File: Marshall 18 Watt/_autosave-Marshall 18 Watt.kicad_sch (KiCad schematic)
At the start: 37 parts, among them J1 LOW, J2 HIGH, J3 Conn_01x03_Socket, J4 Heater, U1 ECC83, U2 ECC83, U3 EL84, U4 EL84

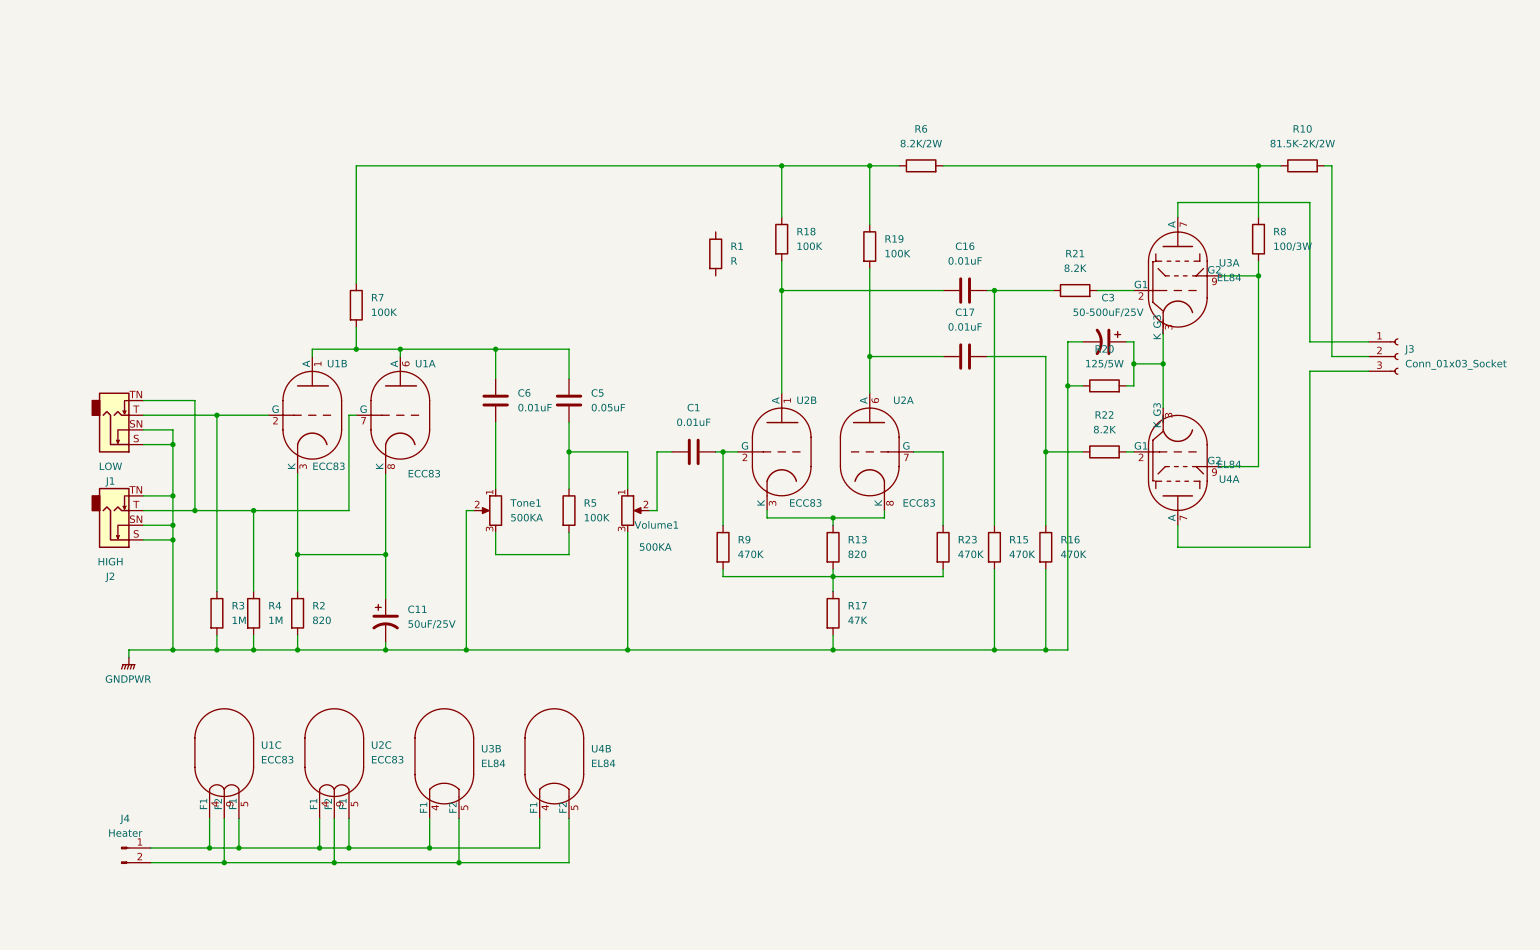
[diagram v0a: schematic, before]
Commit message: Update_17_03_25
Add sch
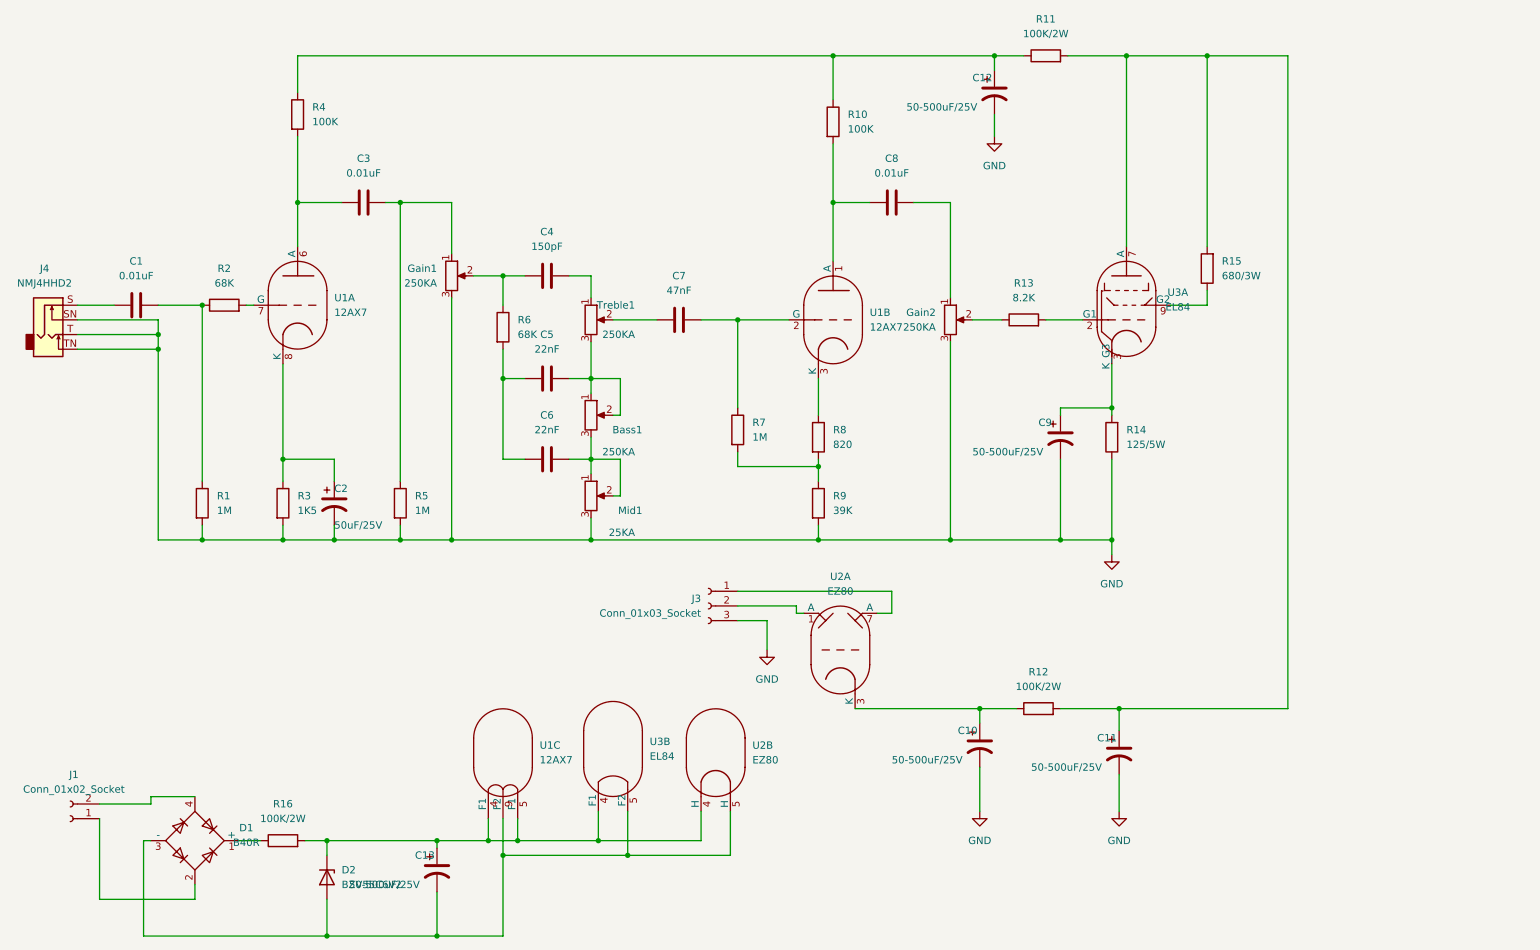
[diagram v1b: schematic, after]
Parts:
- removed C17: 0.01uF, Capacitor_THT:C_Axial_L5.1mm_D3.1mm_P10.00mm_Horizontal, symbol Device:C
- removed J1: LOW, Connector_Audio:Jack_6.35mm_Neutrik_NMJ4HCD2_Horizontal, symbol Connector_Audio:NMJ4HHD2
- removed J2: HIGH, Connector_Audio:Jack_6.35mm_Neutrik_NMJ4HCD2_Horizontal, symbol Connector_Audio:NMJ4HHD2
- removed J4: Heater, Connector_Phoenix_MC_HighVoltage:PhoenixContact_MCV_1,5_2-G-5.08_1x02_P5.08mm_Vertical, symbol Connector:Conn_01x02_Pin
- removed R1: R, Resistor_THT:R_Axial_DIN0411_L9.9mm_D3.6mm_P20.32mm_Horizontal, symbol Device:R
- removed R10: 81.5K-2K/2W, Resistor_THT:R_Axial_DIN0411_L9.9mm_D3.6mm_P20.32mm_Horizontal, symbol Device:R
- removed R15, R23: 470K, Resistor_THT:R_Axial_DIN0411_L9.9mm_D3.6mm_P20.32mm_Horizontal, symbol Device:R
- removed R19: 100K, Resistor_THT:R_Axial_DIN0411_L9.9mm_D3.6mm_P20.32mm_Horizontal, symbol Device:R
- removed R22: 8.2K, Resistor_THT:R_Axial_DIN0411_L9.9mm_D3.6mm_P20.32mm_Horizontal, symbol Device:R
- removed R4: 1M, Resistor_THT:R_Axial_DIN0411_L9.9mm_D3.6mm_P20.32mm_Horizontal, symbol Device:R
- removed U1, U2: ECC83, Valve:Valve_Noval_P, symbol Valve:ECC83
- removed U4: EL84, Valve:Valve_Noval_P, symbol Valve:EL84
- added C1: 0.01uF, Capacitor_THT:C_Axial_L5.1mm_D3.1mm_P10.00mm_Horizontal, symbol Device:C
- added C10, C11, C12, C13: 50-500uF/25V, Capacitor_THT:CP_Radial_D8.0mm_P5.00mm, symbol Device:C_Polarized_US
- added C3: 0.01uF, Capacitor_THT:CP_Radial_D8.0mm_P5.00mm, symbol Device:C
- added C6: 22nF, Capacitor_THT:C_Axial_L5.1mm_D3.1mm_P10.00mm_Horizontal, symbol Device:C
- added D1: B40R, Diode_THT:Diode_Bridge_Round_D9.0mm, symbol Diode_Bridge:B40R
- added D2: BZV55C6V2, Diode_SMD:D_MiniMELF, symbol Diode:BZV55C6V2
- added Gain1, Gain2: 250KA, Potentiometer_THT:Potentiometer_Alps_RK163_Single_Horizontal, symbol Device:R_Potentiometer
- added J1: Conn_01x02_Socket, Connector_PinSocket_2.54mm:PinSocket_1x02_P2.54mm_Vertical, symbol Connector:Conn_01x02_Socket
- added J4: NMJ4HHD2, Connector_Audio:Jack_6.35mm_Neutrik_NMJ4HHD2_Horizontal, symbol Connector_Audio:NMJ4HHD2
- added Mid1: 25KA, Potentiometer_THT:Potentiometer_Alps_RK163_Single_Horizontal, symbol Device:R_Potentiometer
- added R12: 100K/2W, Resistor_THT:R_Axial_DIN0411_L9.9mm_D3.6mm_P20.32mm_Horizontal, symbol Device:R
- added R2: 68K, Resistor_THT:R_Axial_DIN0411_L9.9mm_D3.6mm_P20.32mm_Horizontal, symbol Device:R
- added R5: 1M, Resistor_THT:R_Axial_DIN0411_L9.9mm_D3.6mm_P20.32mm_Horizontal, symbol Device:R
- added U1: 12AX7, Elab:9P_2.57mm, symbol Elab:12AX7
- added U2: EZ80, Valve:Valve_Noval_P, symbol Elab:EZ80
- Bass1: renamed from Volume1; value 500KA -> 250KA
- C4: renamed from C6; value 0.01uF -> 150pF
- C5: value 0.05uF -> 22nF
- C7: renamed from C1; value 0.01uF -> 47nF
- J3: footprint Connector_Phoenix_MC_HighVoltage:PhoenixContact_MCV_1,5_3-G-5.08_1x03_P5.08mm_Vertical -> Connector_Phoenix_MC_HighVoltage:PhoenixContact_MCV_1,5_3-GF-5.08_1x03_P5.08mm_Vertical_ThreadedFlange
- R11: renamed from R6; value 8.2K/2W -> 100K/2W
- R15: renamed from R8; value 100/3W -> 680/3W
- R16: value 470K -> 100K/2W
- R3: renamed from R2; value 820 -> 1K5
- R6: renamed from R5; value 100K -> 68K
- R7: renamed from R9; value 470K -> 1M
- R9: renamed from R17; value 47K -> 39K
- Treble1: renamed from Tone1; value 500KA -> 250KA
- renumbered C11 to C2, C16 to C8, C3 to C9, R3 to R1, R18 to R10, R21 to R13, R20 to R14, R7 to R4, R13 to R8
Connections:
- net at C7.1: now also Treble1.2; no longer Bass1.2
- net at C7.2, R7.1: now also U1.2 (G)
- net at Bass1.1, C5.2: now also Bass1.2, Treble1.3; no longer R6.1
- net at R8.1: now also U1.3 (K)
- net at U3.7 (A): now also R11.2, R15.2, C11.1, R12.2; no longer J3.1 (Pin_1)
- net at J3.2 (Pin_2): now also U2.1 (A)
- net GND: now reaches J3.3 (Pin_3)
- net GND: now also C2.2, C9.2, R1.2, R14.1, R3.2, R9.2, C10.2, C11.2, C12.2, Gain1.3, Gain2.3, J4.SN, J4.T, J4.TN, Mid1.3, R5.2
- net at U3.4 (F1): now also R16.2, C13.1, D2.1 (K), U1.4 (F1), U1.5 (F1), U2.4 (H)
- net at U3.5 (F2): now also C13.2, D1.3 (-), D2.2 (A), U1.9 (F2), U2.5 (H)
- net at R16.1: now also D1.1 (+)
- net at R6.2: now also C5.1, C6.1; no longer Treble1.3
- net at R10.1, R11.1, R4.1: now also C12.1
- net at R1.1: now also C1.2, R2.1
- net at C8.2: now also Gain2.1; no longer R13.1
- net at C8.1, R10.2: now also U1.1 (A)
- net at C2.1, R3.1: now also U1.8 (K)
- removed net GNDPWR: Bass1.3, C2.2, C9.2, R1.2, R14.1, R16.2, R3.2, R9.2, Treble1.2
- new net: C1.1, J4.S
- new net: D1.2, J1.1 (Pin_1)
- new net: D1.4, J1.2 (Pin_2)
- new net: C10.1, R12.1, U2.3 (K)
- new net: C3.1, R4.2, U1.6 (A)
- new net: Bass1.3, C6.2, Mid1.1, Mid1.2
- new net: R2.2, U1.7 (G)
- new net: J3.1 (Pin_1), U2.7 (A)
- new net: Gain2.2, R13.1
- new net: C3.2, Gain1.1, R5.1
- new net: C4.1, Gain1.2, R6.1
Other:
- moved on the sheet: Bass1, C2, C4, C5, C7, C8, C9, R1, R10, R11, R13, R14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
